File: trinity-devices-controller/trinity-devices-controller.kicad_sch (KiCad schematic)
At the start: 90 parts, among them IC1 LM25145RGYR, IC2 MCP2562, J1 xh2pin, J10 xh2pin, J11 Conn_01x03, J12 Conn_01x03, J13 Conn_01x03, J2 xh2pin, J3 Conn_01x01_Pin, J4 Conn_01x01_Pin, J5 Conn_01x04, J6 Conn_01x04, J7 Conn_01x04_Pin, J8 Conn_01x04, J9 xh2pin, Q1 IRFML8244TRPBFTR, Q2 IRFML8244TRPBFTR, Q3 TPH7R506NH,L1Q, Q4 TPH2R306NH1,LQ, Q5 IRFML8244TRPBFTR, Q6 IRFML8244TRPBFTR, SW1 SW_Push, U1 TLP293-4, U3 STM32G431K8Tx, U4 NJM12888F33, U6 NJM7805SDL1, U8 ISO6540FQDBQRQ1

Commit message: 配置、配線完了
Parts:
- added C32: 0.1uf, Capacitor_SMD:C_0603_1608Metric_Pad1.08x0.95mm_HandSolder, symbol Device:C
- added D10, D11, D12, D5, D6, D7, D8, D9: LED, LED_SMD:LED_0603_1608Metric_Pad1.05x0.95mm_HandSolder, symbol Device:LED
- added J14: Conn_01x02, Connector_AMASS:AMASS_XT30UPB-M_1x02_P5.0mm_Vertical, symbol Connector_Generic:Conn_01x02
- added J15: Conn_01x03, Connector_JST:JST_XH_B3B-XH-A_1x03_P2.50mm_Vertical, symbol Connector_Generic:Conn_01x03
- added R27, R28, R29, R30, R31: 10k, Resistor_SMD:R_0603_1608Metric_Pad0.98x0.95mm_HandSolder, symbol Device:R
- added R32, R33, R34, R35, R36, R37, R38, R39: 1k, Resistor_SMD:R_0603_1608Metric_Pad0.98x0.95mm_HandSolder, symbol Device:R
- J1, J10, J2, J9: footprint Connector_JST:JST_XH_S2B-XH-A_1x02_P2.50mm_Horizontal -> Connector_JST:JST_XH_B2B-XH-A_1x02_P2.50mm_Vertical
- J11, J12, J13: footprint Connector_JST:JST_XH_S3B-XH-A_1x03_P2.50mm_Horizontal -> Connector_JST:JST_XH_B3B-XH-A_1x03_P2.50mm_Vertical
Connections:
- net +12V: now also J11.2 (Pin_2), J12.2 (Pin_2), J13.2 (Pin_2), J14.2 (Pin_2), J15.2 (Pin_2); no longer J11.3 (Pin_3), J12.3 (Pin_3), J13.3 (Pin_3)
- net GND: now also C32.2, J14.1 (Pin_1), J15.1 (Pin_1), R27.1, R28.1, R29.1, R30.1
- net GNDD: now also D10.1 (K), D11.1 (K), D12.1 (K), D5.1 (K), D6.1 (K), D7.1 (K), D8.1 (K), D9.1 (K), R31.2
- net IN1: now also U3.10 (PA5), R32.1; no longer U3.9 (PA4)
- net IN2: now also U3.9 (PA4), R33.1; no longer U3.10 (PA5)
- net IN3: now also R34.1
- net IN4: now also R35.1
- net PWM1: now also J11.3 (Pin_3), U8.11 (OUTD), R27.2; no longer J11.2 (Pin_2), U8.14 (OUTA)
- net PWM2: now also J12.3 (Pin_3), U8.12 (OUTC), R28.2; no longer J12.2 (Pin_2), U8.13 (OUTB)
- net PWM3: now also J13.3 (Pin_3), U8.13 (OUTB), R29.2; no longer J13.2 (Pin_2), U8.12 (OUTC)
- net TIM2_CH1: now also U8.6 (IND), R31.1, R39.1; no longer R26.1, U8.3 (INA)
- net TIM2_CH2: now also R24.1, U8.5 (INC), R38.1; no longer R25.1, U8.4 (INB)
- net TIM2_CH3: now also R25.1, U8.4 (INB), R37.1; no longer R24.1, U8.5 (INC)
- net VCC: now also C32.1
- net at R18.2: now also U1.3; no longer U1.5
- net at R3.1, R5.1: now also U1.11; no longer U1.15
- net at R2.2: now also U1.7; no longer U1.3
- net at R4.1, R6.1: now also U1.9; no longer U1.13
- net at U1.1: now also R21.2; no longer R1.2
- net at R19.1, R20.1: now also U1.13; no longer U1.11
- net at C3.2, C5.1, IC1.5 (FB)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: now also R14.2; no longer C6.2
- net at C5.2, IC1.4 (COMP): now also C6.1; no longer R14.1
- net TIM2_CH4: now reaches U3.8 (PA3)
- net TIM2_CH4: now also R26.1, U8.3 (INA), R36.1
- net at R22.1, R23.1: now also U1.15; no longer U1.9
- new net: D8.2 (A), R35.2
- new net: D5.2 (A), R32.2
- new net: D6.2 (A), R33.2
- new net: D10.2 (A), R37.2
- new net: D11.2 (A), R38.2
- new net: D7.2 (A), R34.2
- new net: C6.2, R14.1
- new net: D9.2 (A), R36.2
- new net: D12.2 (A), R39.2
- new net: R1.2, U1.5
- new net PWM4: J15.3 (Pin_3), R30.2, U8.14 (OUTA)
- no-connect marks 17 -> 14
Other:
- note added: "電源入出力"
- note removed: "電源入力"
- moved on the sheet: C6, J11, J12, J13, J3, J4, R14, R24, R25, R26, U1A, U1B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

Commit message: ビア以外完成
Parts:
- added D13, D14, D15, D16, D17: LED, LED_SMD:LED_0603_1608Metric_Pad1.05x0.95mm_HandSolder, symbol Device:LED
- added R40, R41, R42, R43, R44: 1k, Resistor_SMD:R_0603_1608Metric_Pad0.98x0.95mm_HandSolder, symbol Device:R
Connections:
- net +12V: now also R40.1
- net +3.3V: now also R43.1
- net +5P: now also R41.1
- net +5V: now also R44.1
- net GND: now also D13.1 (K), D14.1 (K), D15.1 (K)
- net GNDD: now also D16.1 (K), D17.1 (K)
- net VCC: now also R42.1
- new net: D15.2 (A), R42.2
- new net: D17.2 (A), R44.2
- new net: D16.2 (A), R43.2
- new net: D13.2 (A), R40.2
- new net: D14.2 (A), R41.2
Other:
- note added: "LED"
- moved on the sheet: D10, D11, D12, D5, D6, D7, D8, D9, J5, J6, J7, J8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

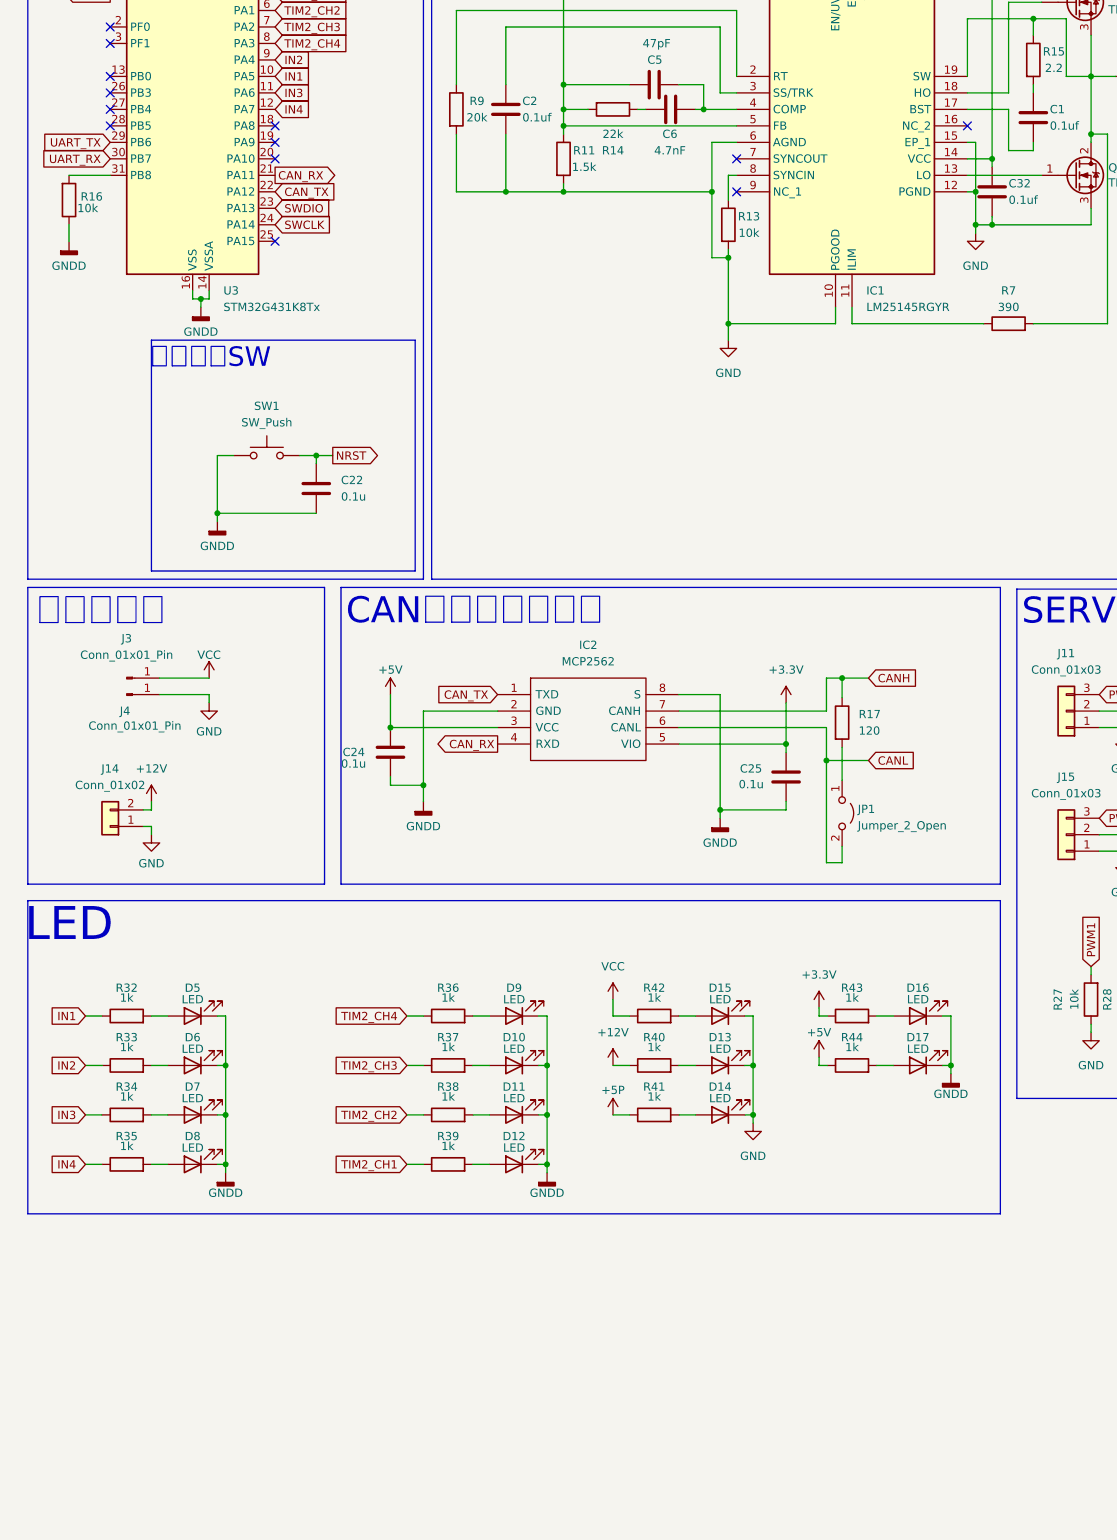
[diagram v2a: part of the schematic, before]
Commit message: 完成、ガーバー作成完了
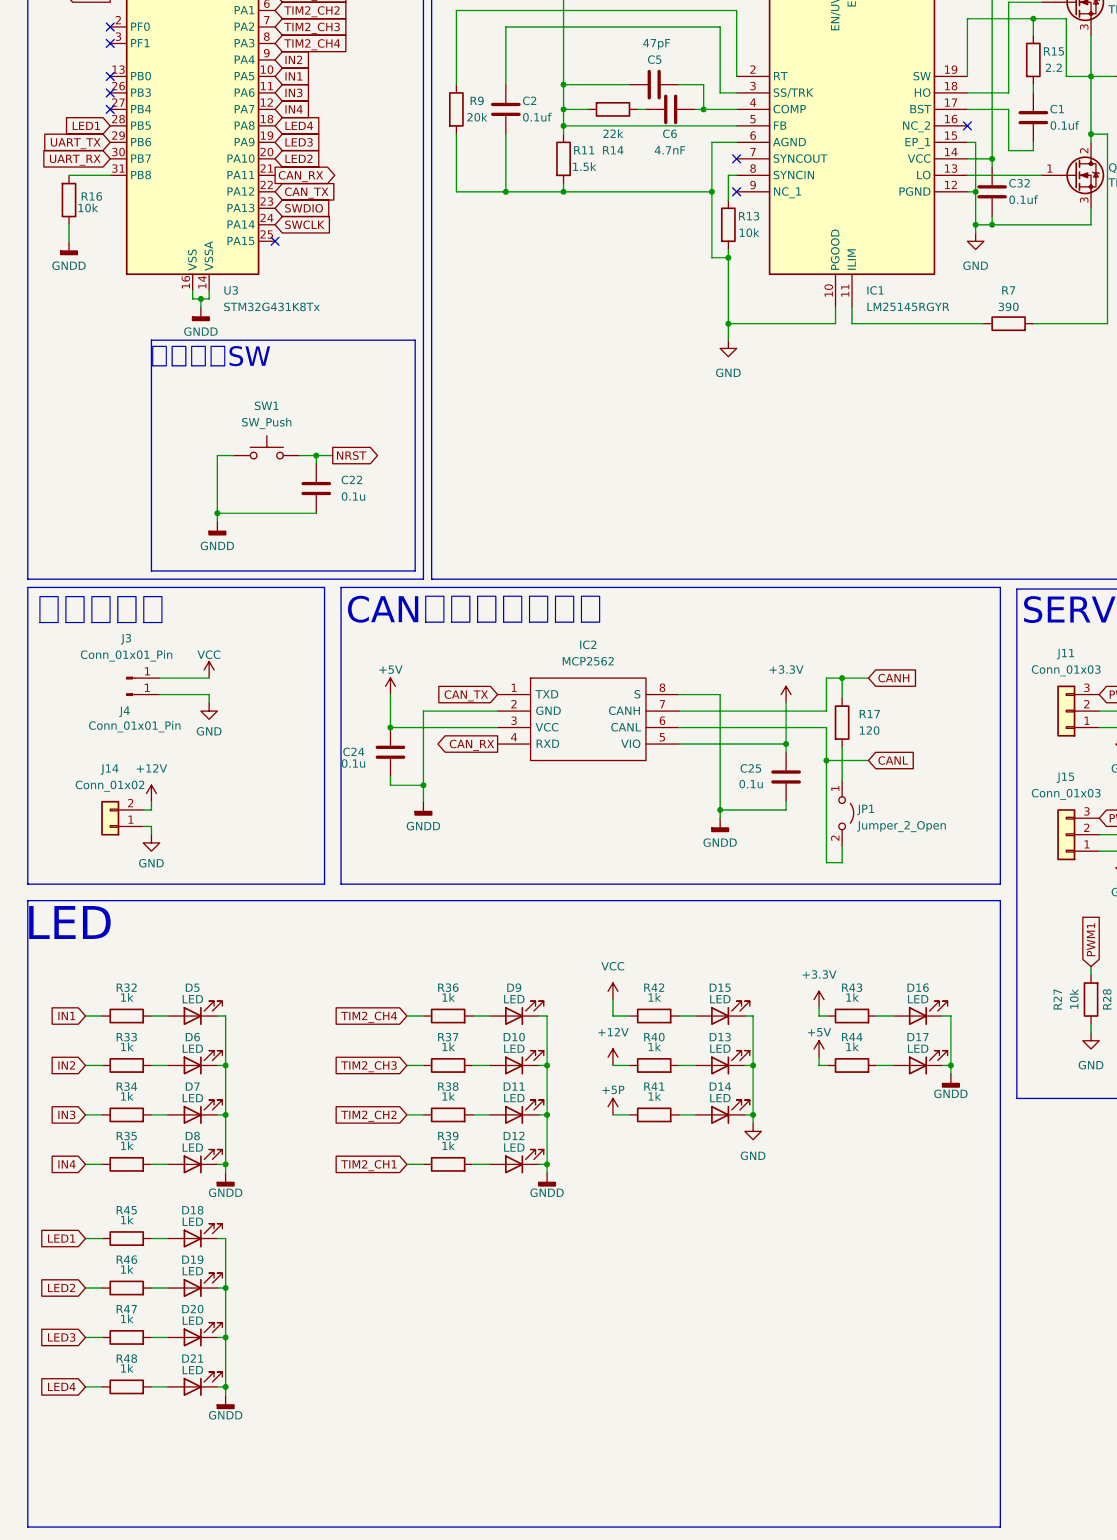
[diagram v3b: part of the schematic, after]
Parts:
- added D18, D19, D20, D21: LED, LED_SMD:LED_0603_1608Metric_Pad1.05x0.95mm_HandSolder, symbol Device:LED
- added R45, R46, R47, R48: 1k, Resistor_SMD:R_0603_1608Metric_Pad0.98x0.95mm_HandSolder, symbol Device:R
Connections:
- net GNDD: now also D18.1 (K), D19.1 (K), D20.1 (K), D21.1 (K)
- net LED4: now reaches U3.18 (PA8)
- net LED4: now also R48.1
- net LED3: now reaches U3.19 (PA9)
- net LED3: now also R47.1
- net LED2: now reaches U3.20 (PA10)
- net LED2: now also R46.1
- net LED1: now reaches U3.28 (PB5)
- net LED1: now also R45.1
- new net: D21.2 (A), R48.2
- new net: D20.2 (A), R47.2
- new net: D18.2 (A), R45.2
- new net: D19.2 (A), R46.2
- no-connect marks 14 -> 10
